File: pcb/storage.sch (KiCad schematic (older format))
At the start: 11 parts, among them Q300 IRLML6402

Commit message: rev 0.1
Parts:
- R301, R302, R303: footprint Resistor_SMD:R_0603_1608Metric -> Resistor_SMD:R_0402_1005Metric
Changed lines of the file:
@@
 F 0 "R301" H 6470 2996 50  0000 L CNN
 F 1 "10K" H 6470 2905 50  0000 L CNN
-F 2 "Resistor_SMD:R_0603_1608Metric" V 6330 2950 50  0001 C CNN
+F 2 "Resistor_SMD:R_0402_1005Metric" V 6330 2950 50  0001 C CNN
 F 3 "~" H 6400 2950 50  0001 C CNN
 	1    6400 2950
@@
 F 0 "R302" H 5970 2996 50  0000 L CNN
 F 1 "10K" H 5970 2905 50  0000 L CNN
-F 2 "Resistor_SMD:R_0603_1608Metric" V 5830 2950 50  0001 C CNN
+F 2 "Resistor_SMD:R_0402_1005Metric" V 5830 2950 50  0001 C CNN
 F 3 "~" H 5900 2950 50  0001 C CNN
 	1    5900 2950
@@
 F 0 "R303" V 6600 3300 50  0000 C CNN
 F 1 "33R" V 6600 3700 50  0000 C CNN
-F 2 "Resistor_SMD:R_0603_1608Metric" V 6580 3500 50  0001 C CNN
+F 2 "Resistor_SMD:R_0402_1005Metric" V 6580 3500 50  0001 C CNN
 F 3 "~" H 6650 3500 50  0001 C CNN
 	1    6650 3500

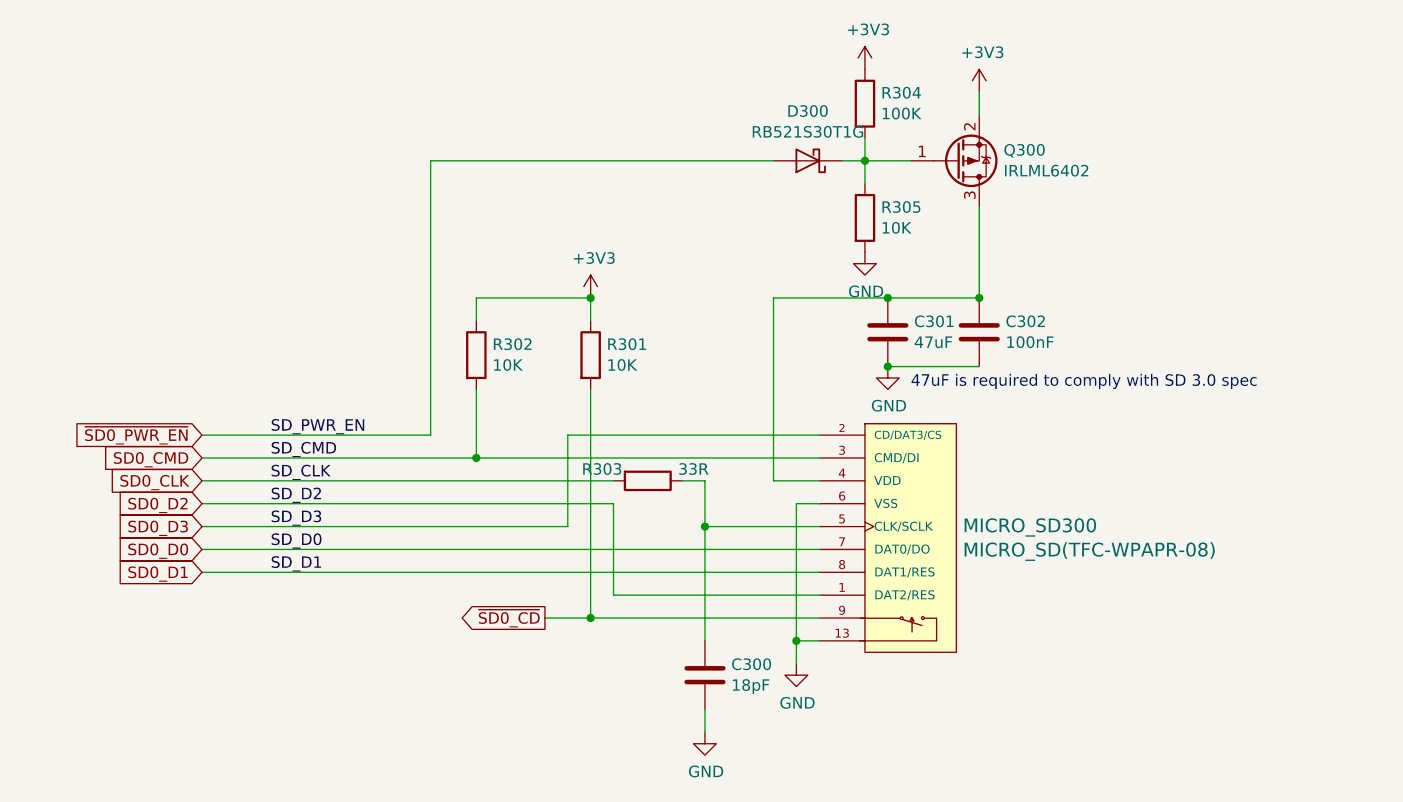
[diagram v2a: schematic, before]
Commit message: pcb: rev 0.2
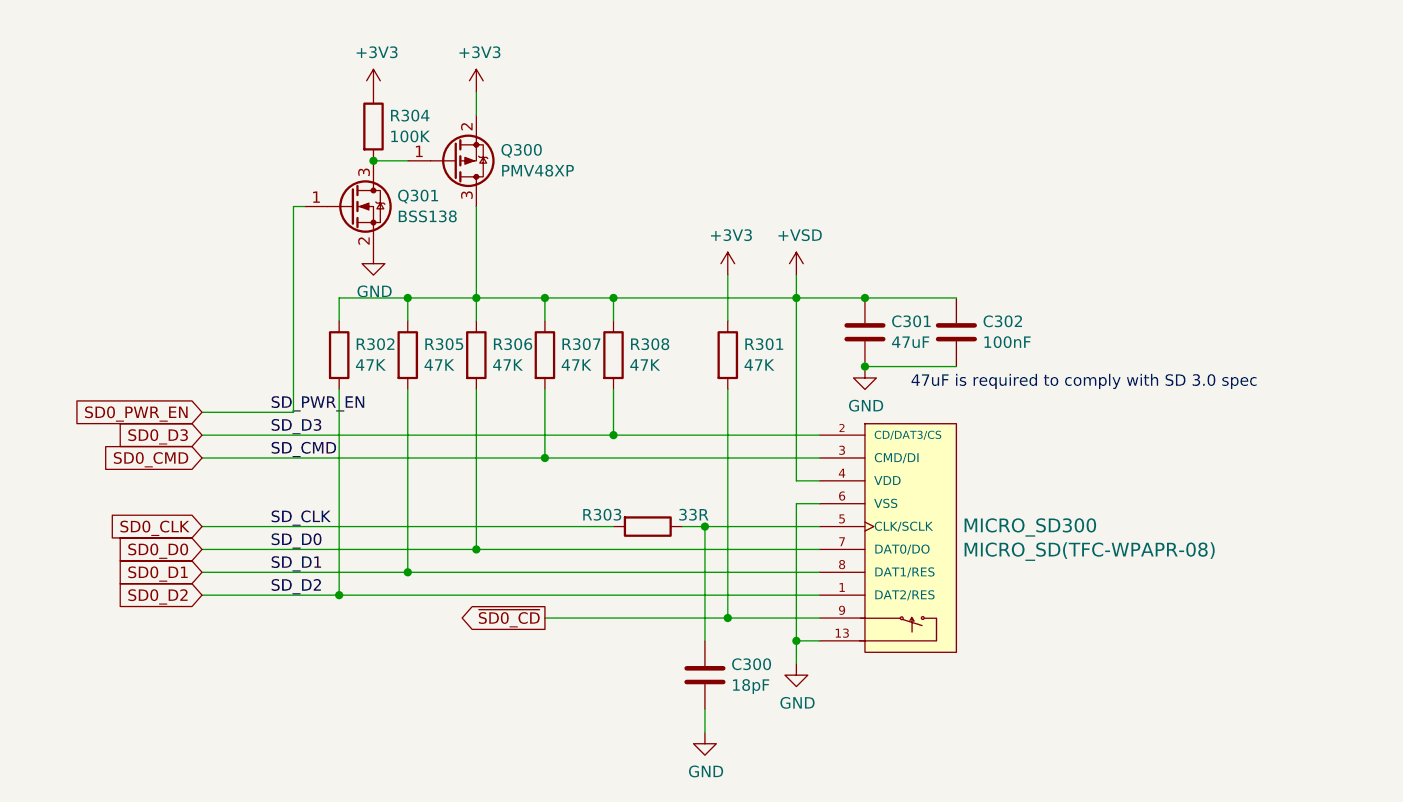
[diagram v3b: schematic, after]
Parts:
- removed D300: RB521S30T1G, Diode_SMD:D_SOD-523, symbol Device:D_Schottky
- added Q301: BSS138, Package_TO_SOT_SMD:SOT-23, symbol Transistor_FET:BSS138
- added R306, R307, R308: 47K, Resistor_SMD:R_0402_1005Metric, symbol Device:R
- Q300: value IRLML6402 -> PMV48XP
- R301, R302: value 10K -> 47K
- R305: value 10K -> 47K; footprint Resistor_SMD:R_0603_1608Metric -> Resistor_SMD:R_0402_1005Metric
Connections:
- net +3V3: no longer R302.1
- net GND: now also Q301.2 (S); no longer R305.2
- net SD0_CMD: now also R307.2; no longer R302.2
- net SD0_D0: now also R306.2
- net SD0_D1: now also R305.2
- net SD0_D2: now also R302.2
- net SD0_D3: now also R308.2
- net at Q300.1 (G), R304.2: now also Q301.3 (D); no longer R305.1
- net +VSD: now reaches C301.1, C302.1, MICRO_SD300.4 (VDD), Q300.3 (D)
- net +VSD: now also R302.1, R305.1, R306.1, R307.1, R308.1
- new net SD0_PWR_EN: Q301.1 (G)
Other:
- moved on the sheet: C301, C302, Q300, R301, R303, R304
